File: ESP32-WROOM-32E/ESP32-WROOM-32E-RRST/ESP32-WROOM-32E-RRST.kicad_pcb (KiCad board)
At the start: 2 copper layers, 115.8 x 100 mm, 76 parts, among them J1 USB_B_Micro, J10 Conn_01x02_Pin, J11 Conn_01x02_Pin, J12 Conn_01x02_Pin, J13 XT60-M, J14 Conn_01x02_Pin, J15 Conn_01x02_Pin, J16 Conn_01x02_Pin, J17 Conn_01x02_Pin, J18 XT60-M, J19 XT60-M, J2 XT60-M, J20 XT60-M, J21 Conn_01x02_Pin, J22 Conn_01x02_Pin, J23 Conn_01x02_Pin, J24 Conn_01x02_Pin, J25 Conn_01x02_Pin, J3 XT60-M, J4 Conn_01x11_Pin, J5 Conn_01x11_Pin, J6 Conn_01x04_Pin, J7 Conn_01x04_Pin, J8 Conn_01x04_Pin, J9 Conn_01x04_Pin, Q1 SS8050-G, Q2 SS8050-G, SW1 SW_Push, SW2 SW_Push, U10 ESP32-WROOM-32E, U11 AMS1117-3.3, U2 MCP2562-E-P, U9 CP2102N-A02-GQFN28

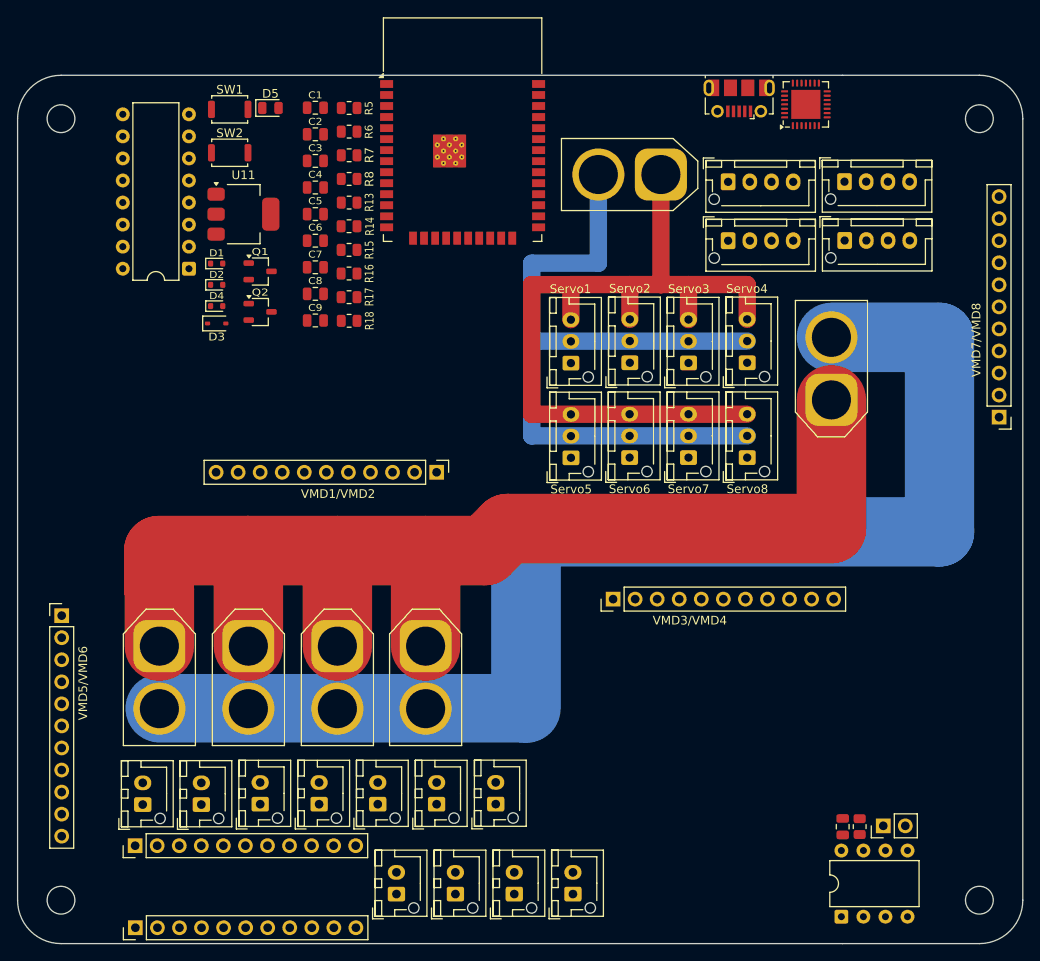
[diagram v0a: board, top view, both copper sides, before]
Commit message: 配線済み
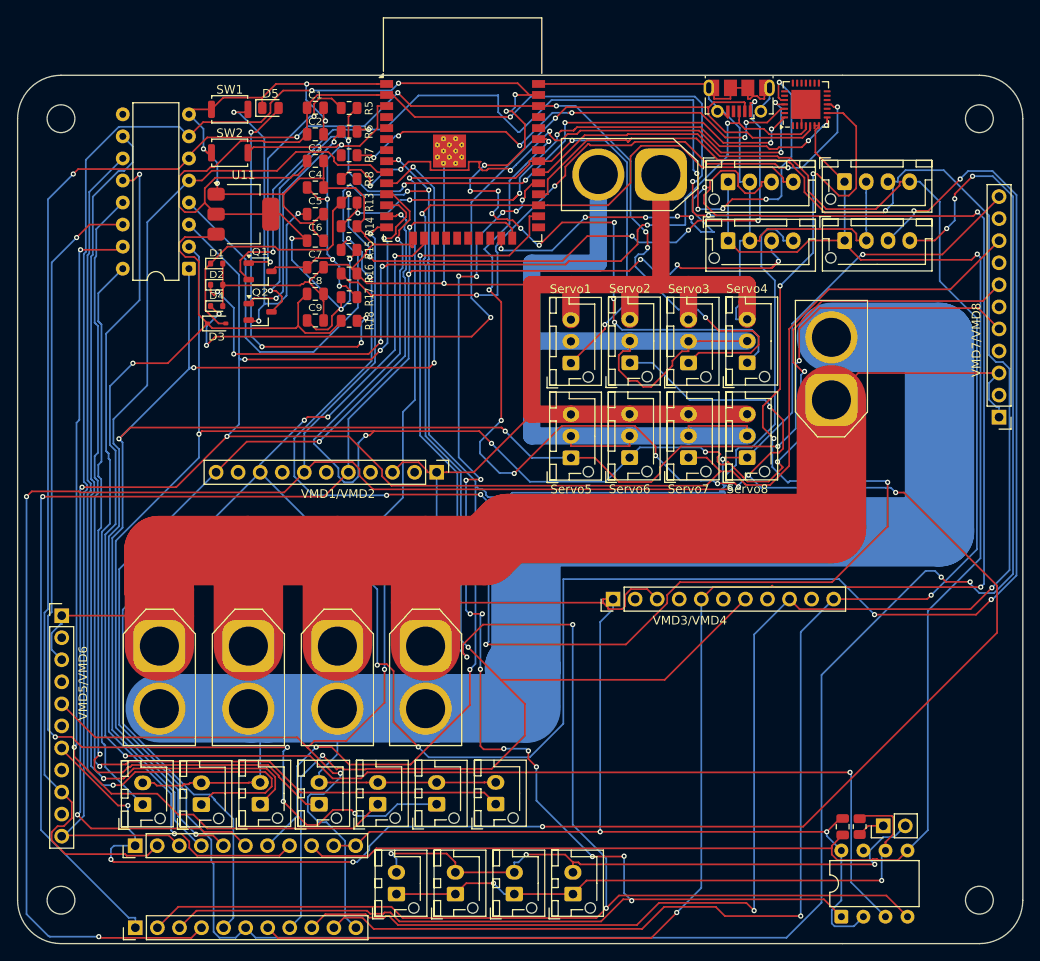
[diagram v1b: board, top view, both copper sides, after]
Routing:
- net GND: track 230.7 -> 718.1 mm, vias 0 -> 7
- net VDD33: track 0.00 -> 347.7 mm, vias 0 -> 7
- net IO13: track 0.00 -> 297.6 mm, vias 0 -> 9
- net IO14: track 0.00 -> 297.4 mm, vias 0 -> 7
- net IO21: track 0.00 -> 282.1 mm, vias 0 -> 14
- net IO27: track 0.00 -> 260.8 mm, vias 0 -> 6
- net IO25: track 0.00 -> 251.4 mm, vias 0 -> 7
- net IO32: track 0.00 -> 248.2 mm, vias 0 -> 7
- net IO26: track 0.00 -> 247.8 mm, vias 0 -> 8
- net IO15: track 0.00 -> 244.3 mm, vias 0 -> 9
- net IO17: track 0.00 -> 228.2 mm, vias 0 -> 3
- net IO23: track 0.00 -> 226.7 mm, vias 0 -> 13
- net IO12: track 0.00 -> 225.7 mm, vias 0 -> 4
- net IO18: track 0.00 -> 210.4 mm, vias 0 -> 2
- net IO22: track 0.00 -> 207.0 mm, vias 0 -> 7
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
